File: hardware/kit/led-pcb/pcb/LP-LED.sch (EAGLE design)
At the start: 2 parts

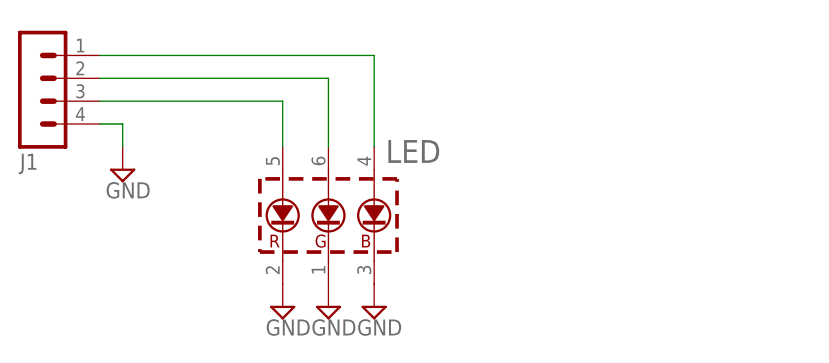
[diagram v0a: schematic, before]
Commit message: rev-b pcb
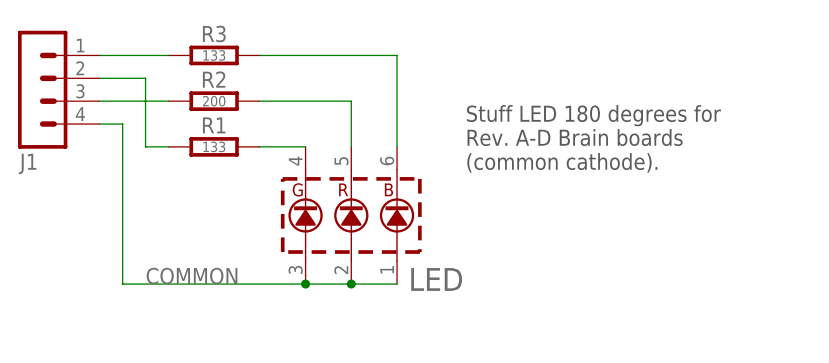
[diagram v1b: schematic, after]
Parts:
- added R1, R3: 133, rlc:RESISTOR0805
- added R2: 200, rlc:RESISTOR0805
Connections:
- removed net GND: J1.4, LED.KB, LED.KG, LED.KR
- new net COMMON: J1.4, LED.AB, LED.AG, LED.AR
- new net N$4: LED.KR, R2.2
- new net N$5: J1.2, R1.1
- new net N$6: J1.1, R3.1
- net N$1: now also LED.KG, R1.2; no longer J1.3, LED.AR
- net N$2: now also J1.3, R2.1; no longer J1.2, LED.AG
- net N$3: now also LED.KB, R3.2; no longer J1.1, LED.AB
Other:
- note added: "Stuff LED 180 degrees for Rev. A-D Brain boards (common cathode)."
- moved on the sheet: LED
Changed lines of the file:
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@@
 <part name="LED" library="led" deviceset="RGB_INDIV" device="PLCC-6"/>
 <part name="J1" library="con-headers" deviceset="MA04-1" device=""/>
-<part name="SUPPLY1" library="supply2" deviceset="GND" device=""/>
-<part name="SUPPLY2" library="supply2" deviceset="GND" device=""/>
-<part name="SUPPLY3" library="supply2" deviceset="GND" device=""/>
-<part name="SUPPLY4" library="supply2" deviceset="GND" device=""/>
+<part name="R2" library="rlc" deviceset="RESISTOR" device="0805" value="200"/>
+<part name="R3" library="rlc" deviceset="RESISTOR" device="0805" value="133"/>
+<part name="R1" library="rlc" deviceset="RESISTOR" device="0805" value="133"/>
 </parts>
 <sheets>
 <sheet>
 <plain>
+<text x="134.62" y="106.68" size="1.778" layer="97">Stuff LED 180 degrees for
+Rev. A-D Brain boards
+(common cathode).</text>
 </plain>
 <instances>
 <instance part="U$1" gate="G$1" x="0" y="0"/>
 <instance part="U$1" gate="G$2" x="76.2" y="0"/>
-<instance part="LED" gate="G$1" x="119.38" y="101.6"/>
+<instance part="LED" gate="G$1" x="121.92" y="101.6" rot="MR180"/>
 <instance part="J1" gate="1" x="86.36" y="114.3" rot="MR180"/>
-<instance part="SUPPLY1" gate="GND" x="96.52" y="106.68"/>
-<instance part="SUPPLY2" gate="GND" x="114.3" y="91.44"/>
-<instance part="SUPPLY3" gate="GND" x="119.38" y="91.44"/>
-<instance part="SUPPLY4" gate="GND" x="124.46" y="91.44"/>
+<instance part="R2" gate="G$1" x="106.68" y="114.3"/>
+<instance part="R3" gate="G$1" x="106.68" y="119.38"/>
+<instance part="R1" gate="G$1" x="106.68" y="109.22"/>
 </instances>
 <busses>
 </busses>
 <nets>
-<net name="GND" class="0">
+<net name="N$3" class="0">
 <segment>
-<pinref part="LED" gate="G$1" pin="KR"/>
-<pinref part="SUPPLY2" gate="GND" pin="GND"/>
+<pinref part="R3" gate="G$1" pin="2"/>
+<wire x1="111.76" y1="119.38" x2="127" y2="119.38" width="0.1524" layer="91"/>
+<pinref part="LED" gate="G$1" pin="KB"/>
+<wire x1="127" y1="119.38" x2="127" y2="109.22" width="0.1524" layer="91"/>
 </segment>
+</net>
+<net name="N$6" class="0">
 <segment>
-<pinref part="LED" gate="G$1" pin="KG"/>
-<pinref part="SUPPLY3" gate="GND" pin="GND"/>
+<pinref part="J1" gate="1" pin="1"/>
+<pinref part="R3" gate="G$1" pin="1"/>
+<wire x1="93.98" y1="119.38" x2="101.6" y2="119.38" width="0.1524" layer="91"/>
 </segment>
+</net>
+<net name="N$5" class="0">
 <segment>
-<pinref part="LED" gate="G$1" pin="KB"/>
-<pinref part="SUPPLY4" gate="GND" pin="GND"/>
+<pinref part="J1" gate="1" pin="2"/>
+<wire x1="93.98" y1="116.84" x2="99.06" y2="116.84" width="0.1524" layer="91"/>
+<wire x1="99.06" y1="116.84" x2="99.06" y2="109.22" width="0.1524" layer="91"/>
+<pinref part="R1" gate="G$1" pin="1"/>
+<wire x1="99.06" y1="109.22" x2="101.6" y2="109.22" width="0.1524" layer="91"/>
 </segment>
+</net>
+<net name="COMMON" class="0">
 <segment>
 <pinref part="J1" gate="1" pin="4"/>
-<pinref part="SUPPLY1" gate="GND" pin="GND"/>
 <wire x1="93.98" y1="111.76" x2="96.52" y2="111.76" width="0.1524" layer="91"/>
-<wire x1="96.52" y1="111.76" x2="96.52" y2="109.22" width="0.1524" layer="91"/>
+<wire x1="96.52" y1="111.76" x2="96.52" y2="93.98" width="0.1524" layer="91"/>
+<label x="99.06" y="93.98" size="1.778" layer="95"/>
+<pinref part="LED" gate="G$1" pin="AB"/>
+<pinref part="LED" gate="G$1" pin="AR"/>
+<wire x1="127" y1="93.98" x2="121.92" y2="93.98" width="0.1524" layer="91"/>
+<pinref part="LED" gate="G$1" pin="AG"/>
+<wire x1="121.92" y1="93.98" x2="116.84" y2="93.98" width="0.1524" layer="91"/>
+<wire x1="116.84" y1="93.98" x2="96.52" y2="93.98" width="0.1524" layer="91"/>
+<junction x="116.84" y="93.98"/>
+<junction x="121.92" y="93.98"/>
 </segment>
 </net>
 <net name="N$1" class="0">
 <segment>
-<pinref part="J1" gate="1" pin="3"/>
-<pinref part="LED" gate="G$1" pin="AR"/>
-<wire x1="93.98" y1="114.3" x2="114.3" y2="114.3" width="0.1524" layer="91"/>
-<wire x1="114.3" y1="114.3" x2="114.3" y2="109.22" width="0.1524" layer="91"/>
+<pinref part="R1" gate="G$1" pin="2"/>
+<pinref part="LED" gate="G$1" pin="KG"/>
+<wire x1="111.76" y1="109.22" x2="116.84" y2="109.22" width="0.1524" layer="91"/>
 </segment>
 </net>
 <net name="N$2" class="0">
 <segment>
-<pinref part="J1" gate="1" pin="2"/>
-<pinref part="LED" gate="G$1" pin="AG"/>
-<wire x1="93.98" y1="116.84" x2="119.38" y2="116.84" width="0.1524" layer="91"/>
-<wire x1="119.38" y1="116.84" x2="119.38" y2="109.22" width="0.1524" layer="91"/>
+<pinref part="J1" gate="1" pin="3"/>
+<pinref part="R2" gate="G$1" pin="1"/>
+<wire x1="93.98" y1="114.3" x2="101.6" y2="114.3" width="0.1524" layer="91"/>
 </segment>
 </net>
-<net name="N$3" class="0">
+<net name="N$4" class="0">
 <segment>
-<pinref part="J1" gate="1" pin="1"/>
-<pinref part="LED" gate="G$1" pin="AB"/>
-<wire x1="93.98" y1="119.38" x2="124.46" y2="119.38" width="0.1524" layer="91"/>
-<wire x1="124.46" y1="119.38" x2="124.46" y2="109.22" width="0.1524" layer="91"/>
+<pinref part="R2" gate="G$1" pin="2"/>
+<pinref part="LED" gate="G$1" pin="KR"/>
+<wire x1="111.76" y1="114.3" x2="121.92" y2="114.3" width="0.1524" layer="91"/>
+<wire x1="121.92" y1="114.3" x2="121.92" y2="109.22" width="0.1524" layer="91"/>
 </segment>
 </net>
@@
 </schematic>
 </drawing>
+<compatibility>
+<note version="6.3" minversion="6.2.2" severity="warning">
+Since Version 6.2.2 text objects can contain more than one line,
+which will not be processed correctly with this version.
+</note>
+</compatibility>
 </eagle>
